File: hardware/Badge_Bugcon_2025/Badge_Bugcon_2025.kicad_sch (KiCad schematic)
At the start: 0 parts

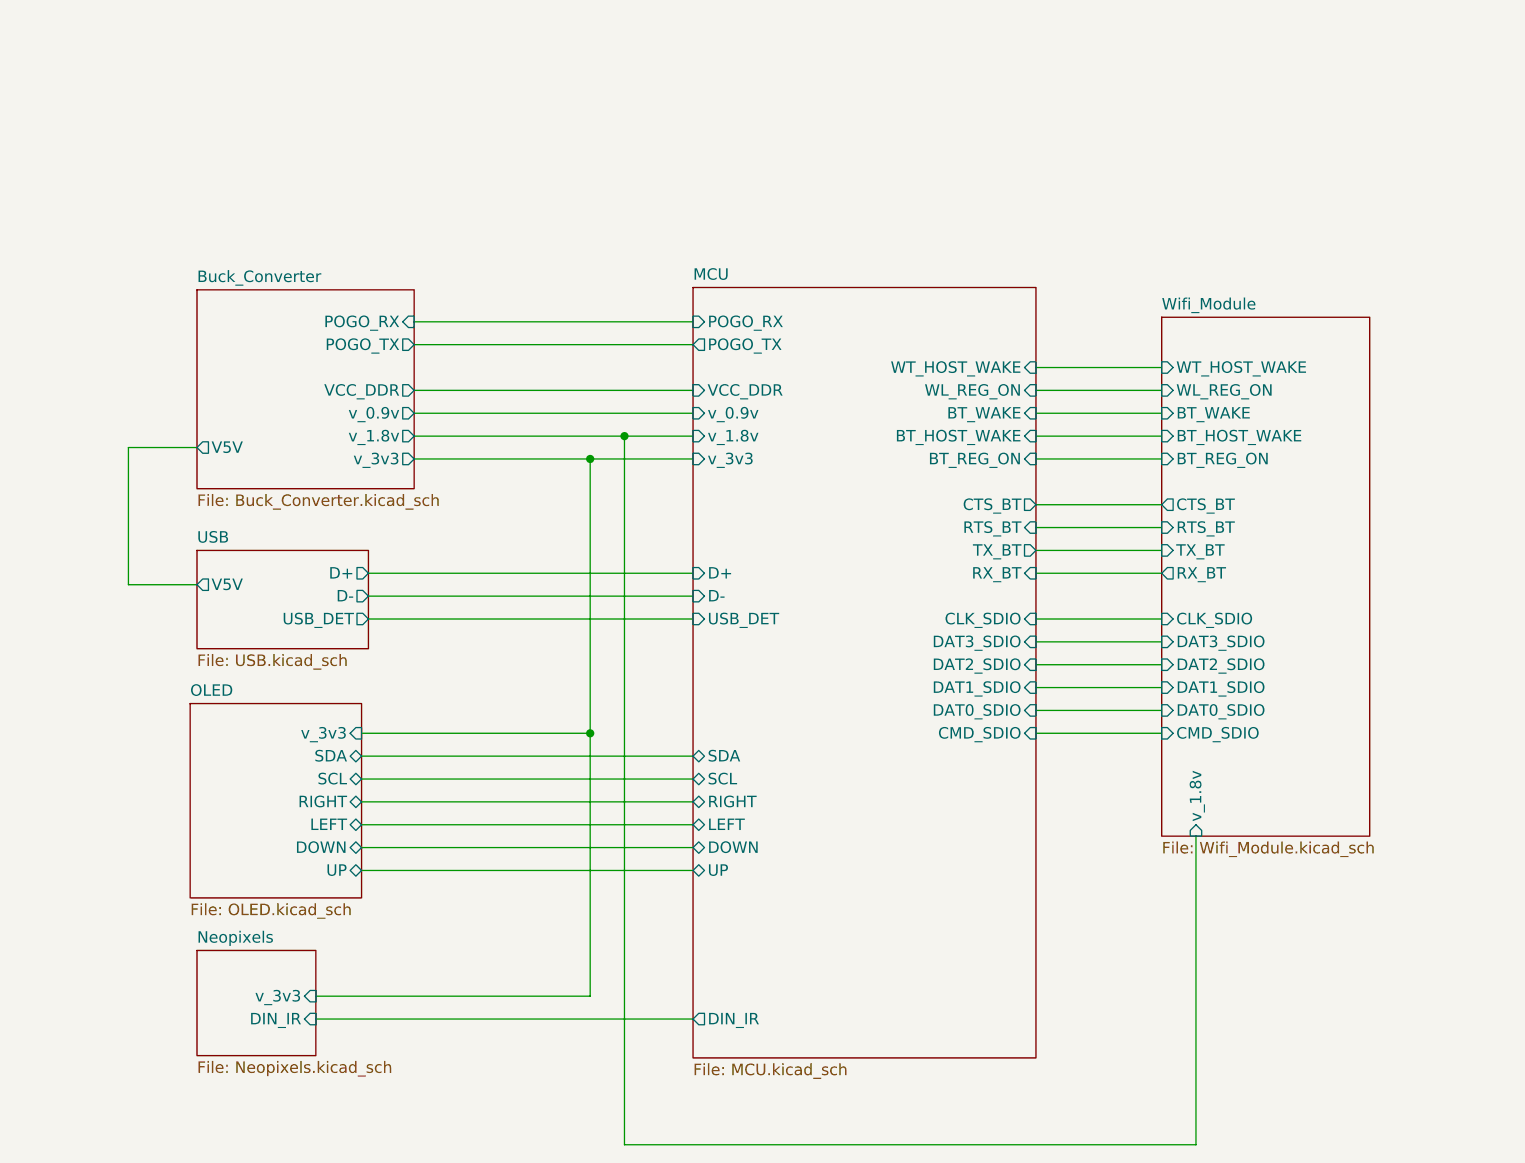
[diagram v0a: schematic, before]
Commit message: feat(Hw):Update_Schematic
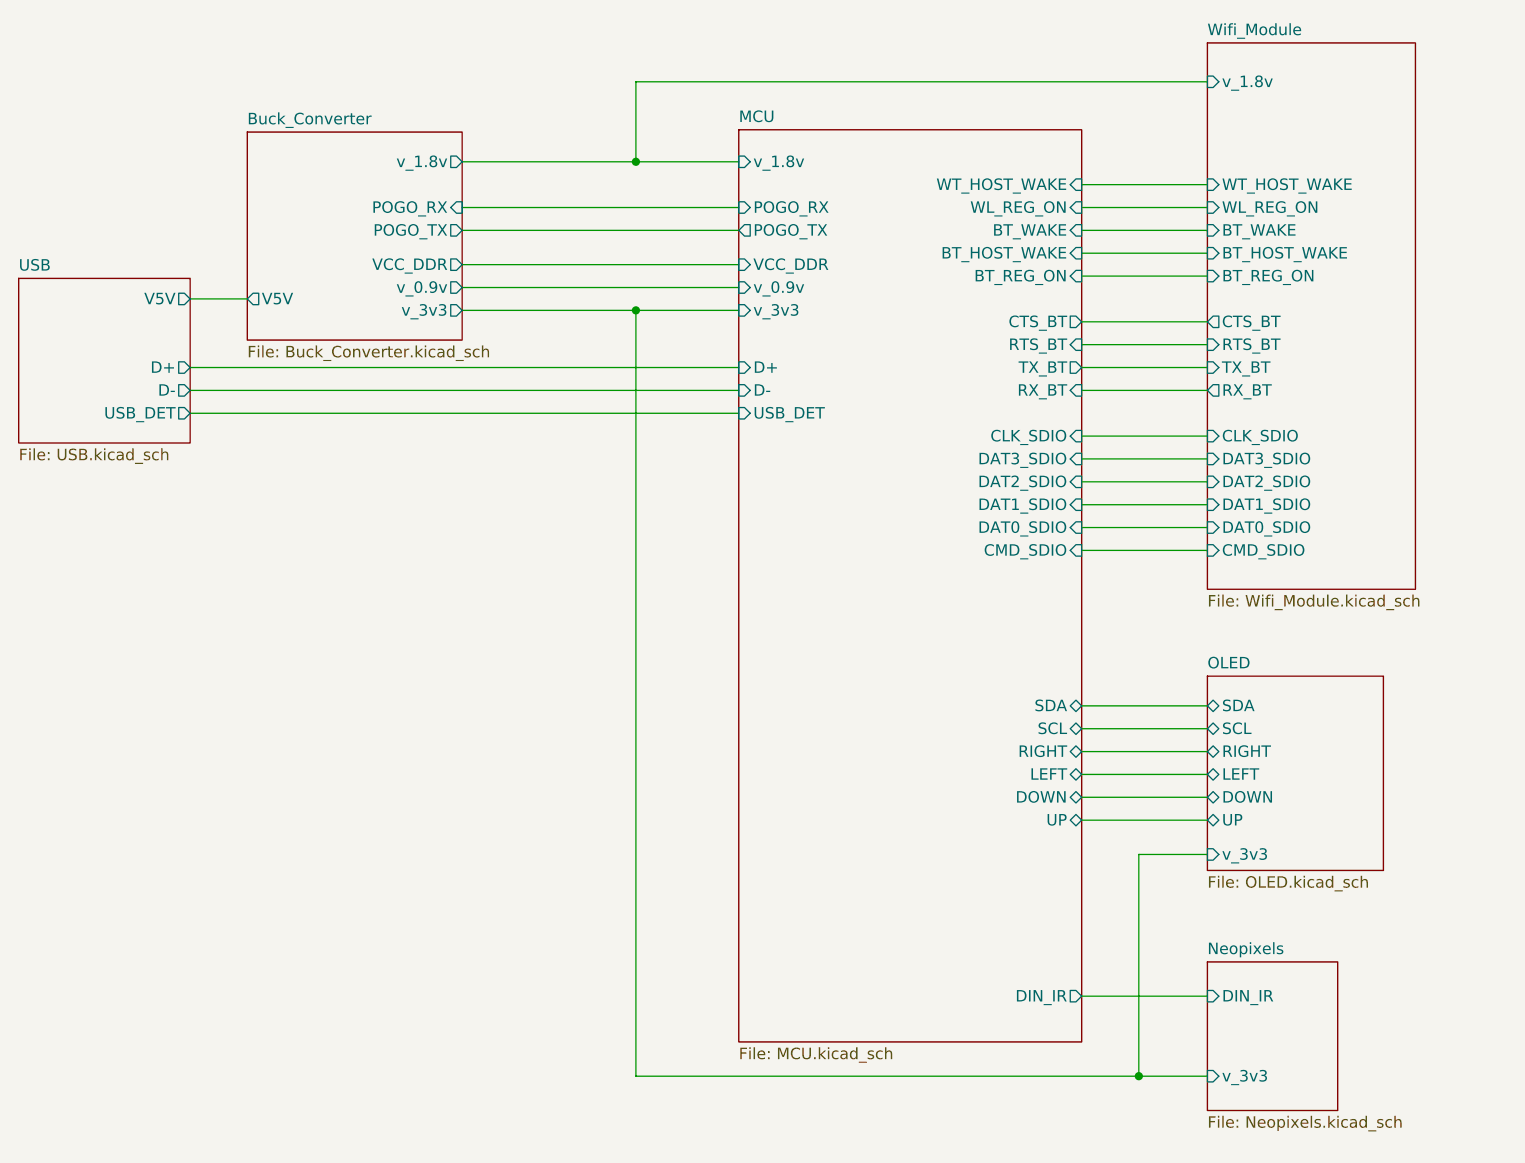
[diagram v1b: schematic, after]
